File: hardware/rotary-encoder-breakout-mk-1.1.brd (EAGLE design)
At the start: 22.9 x 20.3 mm, 3 parts, among them U1 ROTARY_ENCODER_SWITCH

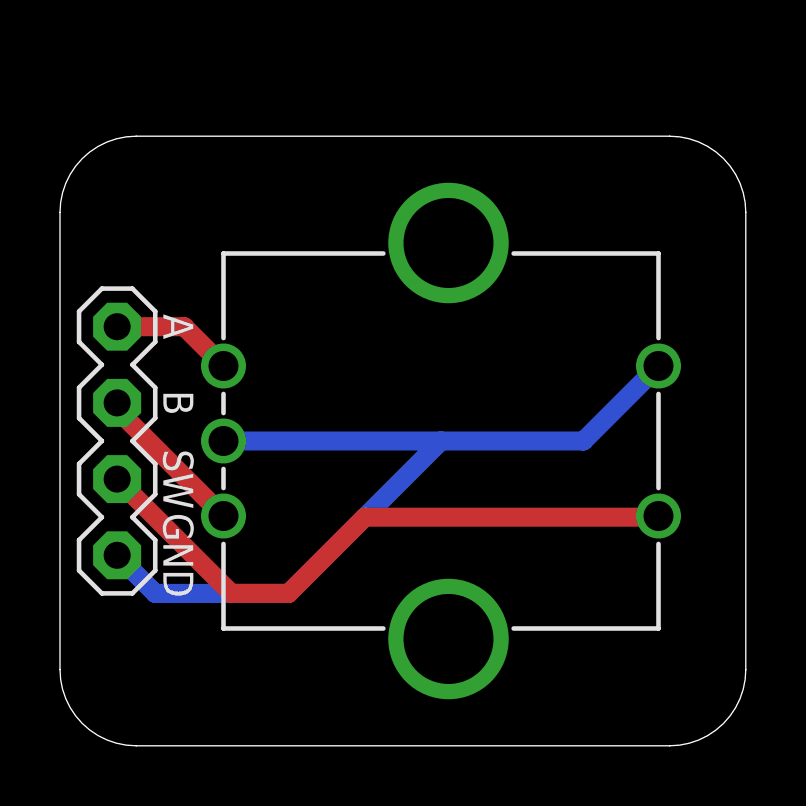
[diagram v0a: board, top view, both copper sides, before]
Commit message: marked up for fab
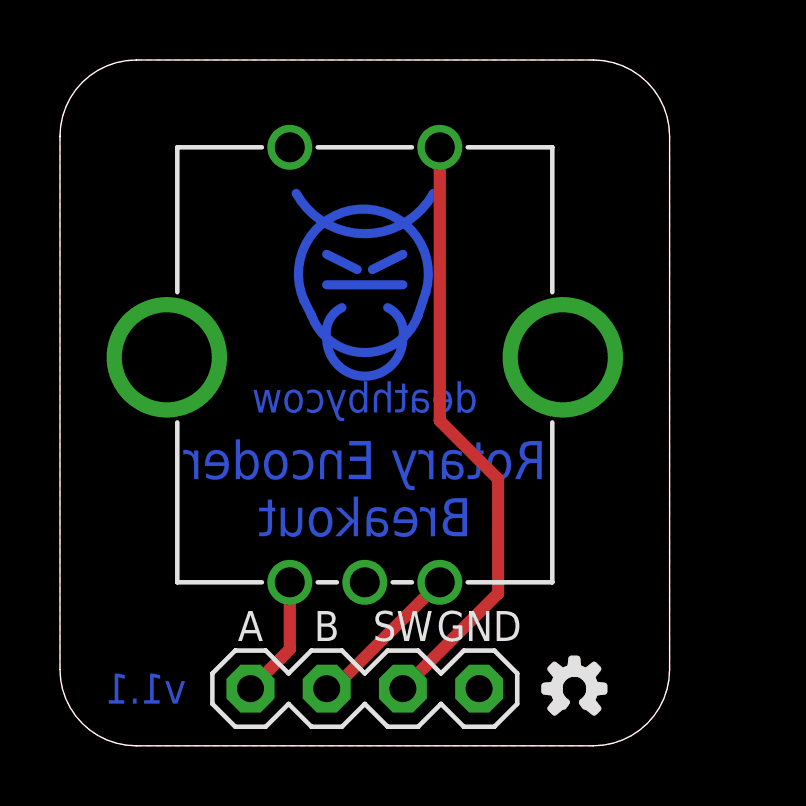
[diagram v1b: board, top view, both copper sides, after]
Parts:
- added U$1, U$3: (no value), A_butts:OSHWLOGO_TINY
- added U$2: (no value), A_butts:COW_SMALL_METAL
- moved JP1 12.9 mm to (14.0, 1.91), turned to 180 degrees
- moved U1 3.59 mm to (10.2, 12.7), turned to 270 degrees
- turned FRAME1 to 90 degrees
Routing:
- net GND: track 29.0 -> 0.00 mm
- net SW1: track 20.7 -> 20.2 mm
- added copper zone on layer 1, net GND
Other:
- board size 22.9 x 20.3 mm -> 20.3 x 22.9 mm
- board text added: ">VERSION"
- board text added: "Rotary Encoder Breakout"
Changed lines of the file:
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@@
 <setting verticaltext="up"/>
 </settings>
-<grid distance="25" unitdist="mil" unit="mil" style="lines" multiple="2" display="yes" altdistance="1" altunitdist="mil" altunit="mil"/>
+<grid distance="12.5" unitdist="mil" unit="mil" style="lines" multiple="2" display="yes" altdistance="1" altunitdist="mil" altunit="mil"/>
 <layers>
 <layer number="1" name="Top" color="4" fill="1" visible="yes" active="yes"/>
@@
 <board>
 <plain>
-<wire x1="0" y1="17.78" x2="0" y2="2.54" width="0" layer="20"/>
+<wire x1="2.54" y1="0" x2="17.78" y2="0" width="0" layer="20"/>
+<wire x1="17.78" y1="0" x2="20.32" y2="2.54" width="0" layer="20" curve="90"/>
+<wire x1="20.32" y1="2.54" x2="20.32" y2="20.32" width="0" layer="20"/>
+<wire x1="20.32" y1="20.32" x2="17.78" y2="22.86" width="0" layer="20" curve="90"/>
+<wire x1="17.78" y1="22.86" x2="2.54" y2="22.86" width="0" layer="20"/>
+<wire x1="2.54" y1="22.86" x2="0" y2="20.32" width="0" layer="20" curve="90"/>
+<wire x1="0" y1="20.32" x2="0" y2="2.54" width="0" layer="20"/>
 <wire x1="0" y1="2.54" x2="2.54" y2="0" width="0" layer="20" curve="90"/>
-<wire x1="2.54" y1="0" x2="20.32" y2="0" width="0" layer="20"/>
-<wire x1="20.32" y1="0" x2="22.86" y2="2.54" width="0" layer="20" curve="90"/>
-<wire x1="22.86" y1="2.54" x2="22.86" y2="17.78" width="0" layer="20"/>
-<wire x1="22.86" y1="17.78" x2="20.32" y2="20.32" width="0" layer="20" curve="90"/>
-<wire x1="20.32" y1="20.32" x2="2.54" y2="20.32" width="0" layer="20"/>
-<wire x1="2.54" y1="20.32" x2="0" y2="17.78" width="0" layer="20" curve="90"/>
-<text x="6.985" y="12.7" size="1" layer="22" font="vector" ratio="12" rot="SMR270" align="top-center">A</text>
-<text x="6.985" y="7.62" size="1" layer="22" font="vector" ratio="12" rot="SMR270" align="top-center">B</text>
-<text x="6.985" y="10.16" size="1" layer="22" font="vector" ratio="12" rot="SMR270" align="top-center">COM</text>
-<text x="18.415" y="7.62" size="1" layer="22" font="vector" ratio="12" rot="SMR90" align="top-center">SW</text>
-<text x="18.415" y="12.7" size="1" layer="22" font="vector" ratio="12" rot="SMR90" align="top-center">COM</text>
-<text x="4.445" y="13.97" size="1" layer="21" font="vector" ratio="12" rot="SR270" align="top-center">A</text>
-<text x="4.445" y="6.35" size="1" layer="21" font="vector" ratio="12" rot="SR270" align="top-center">GND</text>
-<text x="4.445" y="11.43" size="1" layer="21" font="vector" ratio="12" rot="SR270" align="top-center">B</text>
-<text x="4.445" y="8.89" size="1" layer="21" font="vector" ratio="12" rot="SR270" align="top-center">SW</text>
+<text x="7.62" y="4.445" size="1" layer="22" font="vector" ratio="12" rot="MR180" align="bottom-center">A</text>
+<text x="12.7" y="4.445" size="1" layer="22" font="vector" ratio="12" rot="MR180" align="bottom-center">B</text>
+<text x="10.16" y="4.445" size="1" layer="22" font="vector" ratio="12" rot="MR180" align="bottom-center">COM</text>
+<text x="12.7" y="20.955" size="1" layer="22" font="vector" ratio="12" rot="MR180" align="top-center">SW</text>
+<text x="7.62" y="20.955" size="1" layer="22" font="vector" ratio="12" rot="MR180" align="top-center">COM</text>
+<text x="6.35" y="3.4925" size="1" layer="21" font="vector" ratio="12" rot="SR0" align="bottom-center">A</text>
+<text x="13.97" y="3.4925" size="1" layer="21" font="vector" ratio="12" rot="SR0" align="bottom-center">GND</text>
+<text x="8.89" y="3.4925" size="1" layer="21" font="vector" ratio="12" rot="SR0" align="bottom-center">B</text>
+<text x="11.43" y="3.4925" size="1" layer="21" font="vector" ratio="12" rot="SR0" align="bottom-center">SW</text>
+<text x="2.8575" y="1.905" size="1" layer="16" font="vector" ratio="16" rot="MR0" align="center">&gt;VERSION</text>
+<text x="2.8575" y="1.905" size="1" layer="22" font="vector" ratio="16" rot="MR0" align="center">&gt;VERSION</text>
+<text x="10.16" y="8.5725" size="1.27" layer="22" font="vector" ratio="15" rot="MR0" align="center">Rotary Encoder
+Breakout</text>
+<text x="10.16" y="8.5725" size="1.27" layer="16" font="vector" ratio="15" rot="MR0" align="center">Rotary Encoder
+Breakout</text>
+<text x="3.175" y="1.905" size="1" layer="1" font="vector" ratio="16" rot="SR0" align="center">&gt;VERSION</text>
+<text x="3.175" y="1.905" size="1" layer="21" font="vector" ratio="16" rot="SR0" align="center">&gt;VERSION</text>
 </plain>
 <attributes>
+<attribute name="VERSION" value="v1.1"/>
 </attributes>
 <variantdefs>
@@
 </autorouter>
 <elements>
-<element name="FRAME1" library="A_butts" package="DUMMY" value="FRAME-LETTERNO_PACKAGE" x="0" y="0">
-<attribute name="VERSION" value="1.0" x="13.97" y="-1.27" size="1.778" layer="27" display="off"/>
-<attribute name="DESIGNER" value="sean@yak.net" x="13.97" y="-1.27" size="1.778" layer="27" display="off"/>
+<element name="FRAME1" library="A_butts" package="DUMMY" value="FRAME-LETTERNO_PACKAGE" x="0" y="0" rot="R90">
+<attribute name="VERSION" value="1.0" x="1.27" y="13.97" size="1.778" layer="27" rot="R90" display="off"/>
+<attribute name="DESIGNER" value="sean@yak.net" x="1.27" y="13.97" size="1.778" layer="27" rot="R90" display="off"/>
 </element>
-<element name="U1" library="A_butts" package="ROTARY_ENCODER_SWITCH" value="ROTARY_ENCODER_SWITCH" x="12.7" y="10.16" smashed="yes" rot="R180"/>
-<element name="JP1" library="A_butts" package="1X04-PTH-VERT" value="M04PTH" x="1.905" y="6.35" smashed="yes" rot="R90"/>
+<element name="U1" library="A_butts" package="ROTARY_ENCODER_SWITCH" value="ROTARY_ENCODER_SWITCH" x="10.16" y="12.7" smashed="yes" rot="R270"/>
+<element name="JP1" library="A_butts" package="1X04-PTH-VERT" value="M04PTH" x="13.97" y="1.905" smashed="yes" rot="R180"/>
+<element name="U$2" library="A_butts" package="COW_SMALL_METAL" value="" x="10.16" y="15.875" rot="MR0"/>
+<element name="U$1" library="A_butts" package="OSHWLOGO_TINY" value="" x="17.145" y="1.905"/>
+<element name="U$3" library="A_butts" package="OSHWLOGO_TINY" value="" x="17.145" y="1.905" rot="MR0"/>
 </elements>
 <signals>
@@
 <contactref element="U1" pad="SW1"/>
 <contactref element="JP1" pad="2"/>
-<wire x1="1.905" y1="8.89" x2="5.715" y2="5.08" width="0.635" layer="1"/>
-<wire x1="5.715" y1="5.08" x2="7.62" y2="5.08" width="0.635" layer="1"/>
-<wire x1="7.62" y1="5.08" x2="10.16" y2="7.62" width="0.635" layer="1"/>
-<wire x1="10.16" y1="7.62" x2="19.91" y2="7.62" width="0.635" layer="1"/>
-<wire x1="19.91" y1="7.62" x2="19.95" y2="7.66" width="0.635" layer="1"/>
+<wire x1="11.43" y1="1.905" x2="14.605" y2="5.08" width="0.4064" layer="1"/>
+<wire x1="14.605" y1="5.08" x2="14.605" y2="8.89" width="0.4064" layer="1"/>
+<wire x1="14.605" y1="8.89" x2="12.66" y2="10.835" width="0.4064" layer="1"/>
+<wire x1="12.66" y1="10.835" x2="12.66" y2="19.95" width="0.4064" layer="1"/>
 </signal>
 <signal name="A">
 <contactref element="U1" pad="A"/>
 <contactref element="JP1" pad="4"/>
-<wire x1="1.905" y1="13.97" x2="4.14" y2="13.97" width="0.635" layer="1"/>
-<wire x1="4.14" y1="13.97" x2="5.45" y2="12.66" width="0.635" layer="1"/>
+<wire x1="6.35" y1="1.905" x2="7.66" y2="3.215" width="0.4064" layer="1"/>
+<wire x1="7.66" y1="3.215" x2="7.66" y2="5.45" width="0.4064" layer="1"/>
 </signal>
 <signal name="B">
 <contactref element="U1" pad="B"/>
 <contactref element="JP1" pad="3"/>
-<wire x1="1.905" y1="11.43" x2="1.905" y2="11.205" width="0.635" layer="1"/>
-<wire x1="1.905" y1="11.205" x2="5.45" y2="7.66" width="0.635" layer="1"/>
+<wire x1="8.89" y1="1.905" x2="9.115" y2="1.905" width="0.4064" layer="1"/>
+<wire x1="9.115" y1="1.905" x2="12.66" y2="5.45" width="0.4064" layer="1"/>
 </signal>
 <signal name="GND">
@@
 <contactref element="U1" pad="SW2"/>
 <contactref element="JP1" pad="1"/>
-<wire x1="1.905" y1="6.35" x2="3.175" y2="5.08" width="0.635" layer="16"/>
-<wire x1="3.175" y1="5.08" x2="7.62" y2="5.08" width="0.635" layer="16"/>
-<wire x1="7.62" y1="5.08" x2="12.7" y2="10.16" width="0.635" layer="16"/>
-<wire x1="12.7" y1="10.16" x2="17.45" y2="10.16" width="0.635" layer="16"/>
-<wire x1="17.45" y1="10.16" x2="19.95" y2="12.66" width="0.635" layer="16"/>
-<wire x1="5.45" y1="10.16" x2="12.7" y2="10.16" width="0.635" layer="16"/>
+<polygon width="0.1524" layer="1">
+<vertex x="20.32" y="20.32"/>
+<vertex x="20.32" y="2.54" curve="-90"/>
+<vertex x="17.78" y="0"/>
+<vertex x="2.54" y="0" curve="-90"/>
+<vertex x="0" y="2.54"/>
+<vertex x="0" y="20.32" curve="-90"/>
+<vertex x="2.54" y="22.86"/>
+<vertex x="17.78" y="22.86" curve="-90"/>
+</polygon>
 </signal>
 </signals>
 </board>
 </drawing>
+<compatibility>
+<note version="6.3" minversion="6.2.2" severity="warning">
+Since Version 6.2.2 text objects can contain more than one line,
+which will not be processed correctly with this version.
+</note>
+</compatibility>
 </eagle>
